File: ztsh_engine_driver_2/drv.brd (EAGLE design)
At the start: 125.7 x 80.9 mm, 57 parts, among them IC1 74AC14N, Q1 IRF640N, Q2 IRF640N, Q3 IRF640N, Q4 IRF640N, U1 IR2110-1PBF, U2 IR2110-1PBF

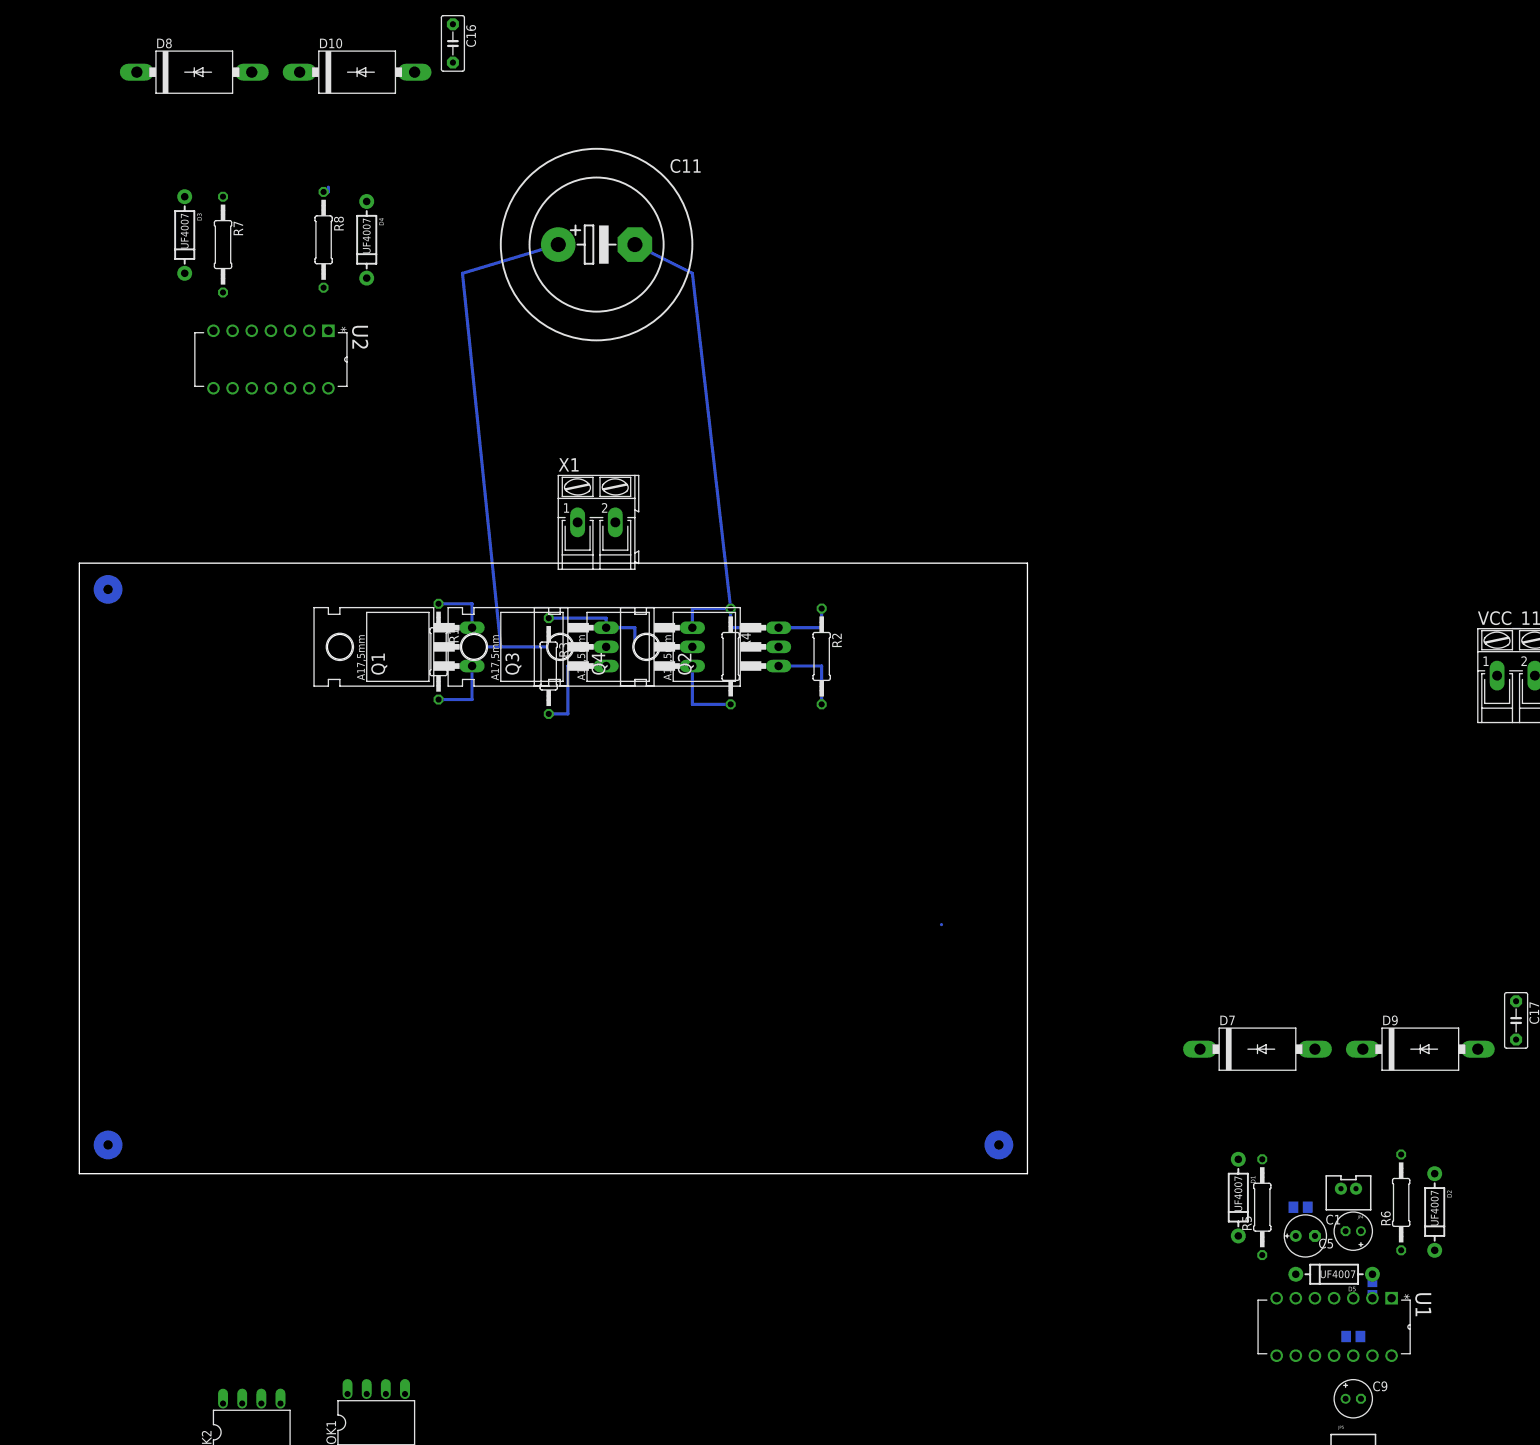
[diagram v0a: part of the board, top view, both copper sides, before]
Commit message: board update...
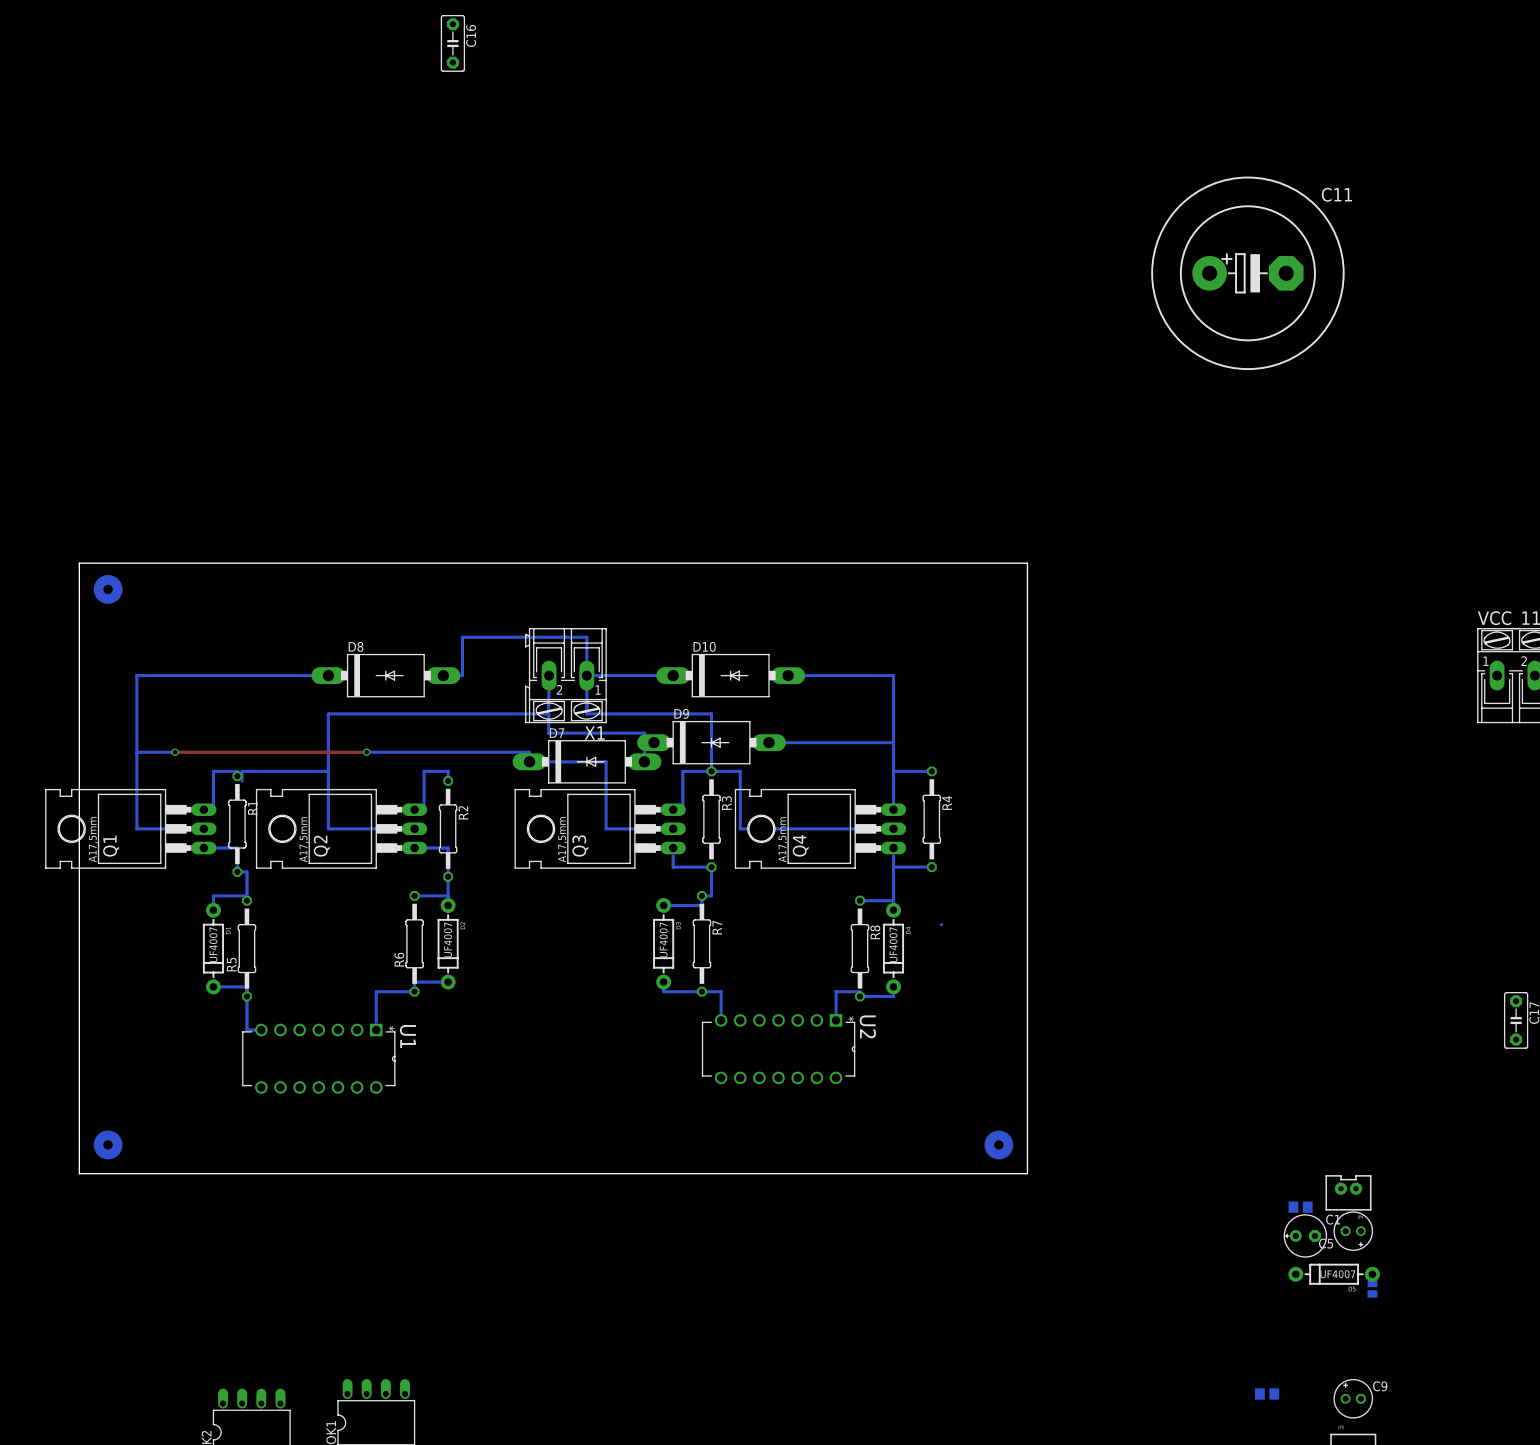
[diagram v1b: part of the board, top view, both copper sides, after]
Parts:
- moved D1 139.8 mm to (17.8, 90.8)
- moved U1 139.2 mm to (24.1, 72.4)
- moved R5 138.9 mm to (22.2, 90.8)
- moved D2 135.6 mm to (48.9, 91.4)
- moved R6 135.2 mm to (44.5, 91.4)
- moved R8 117.9 mm to (103.5, 90.8)
- moved D4 117.1 mm to (108.0, 90.8)
- moved U2 113.5 mm to (85.1, 73.7)
- moved D3 113.4 mm to (77.5, 91.4)
- moved R7 112.4 mm to (82.5, 91.4)
- moved D9 102.4 mm to (83.8, 118.1)
- moved D7 96.7 mm to (67.3, 115.6)
- moved D10 94.1 mm to (86.4, 127.0)
- moved C11 86.4 mm to (154.9, 180.3)
- moved D8 83.9 mm to (40.6, 127.0)
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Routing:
- net OUT2: track 7.62 -> 104.1 mm
- net OUT1: track 22.9 -> 111.8 mm
- net VCC_110: track 80.8 -> 135.9 mm, vias 0 -> 2
- net N$7: track 0.00 -> 15.9 mm
- net AGND: track 78.0 -> 64.2 mm
- net N$11: track 0.00 -> 13.3 mm
- net N$10: track 0.00 -> 12.7 mm
- net N$5: track 0.00 -> 12.1 mm
- net N$1: track 8.89 -> 19.7 mm
- net N$4: track 10.8 -> 17.8 mm
- net N$14: track 11.4 -> 17.8 mm
- net N$9: track 14.0 -> 19.0 mm
